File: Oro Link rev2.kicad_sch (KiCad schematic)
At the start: 18 parts, among them J1 690357100872, J10 690367180872, J11 690367180872, J12 690367180872, J13 690367180872, J14 690357100872, J15 690357100872, J16 690357100872, J17 690357100872, J18 690357100872, J2 690357100872, J3 690357100872, J4 690357100872, J5 690367180872, J6 690367180872, J7 690367180872, J8 690367180872, J9 690367180872

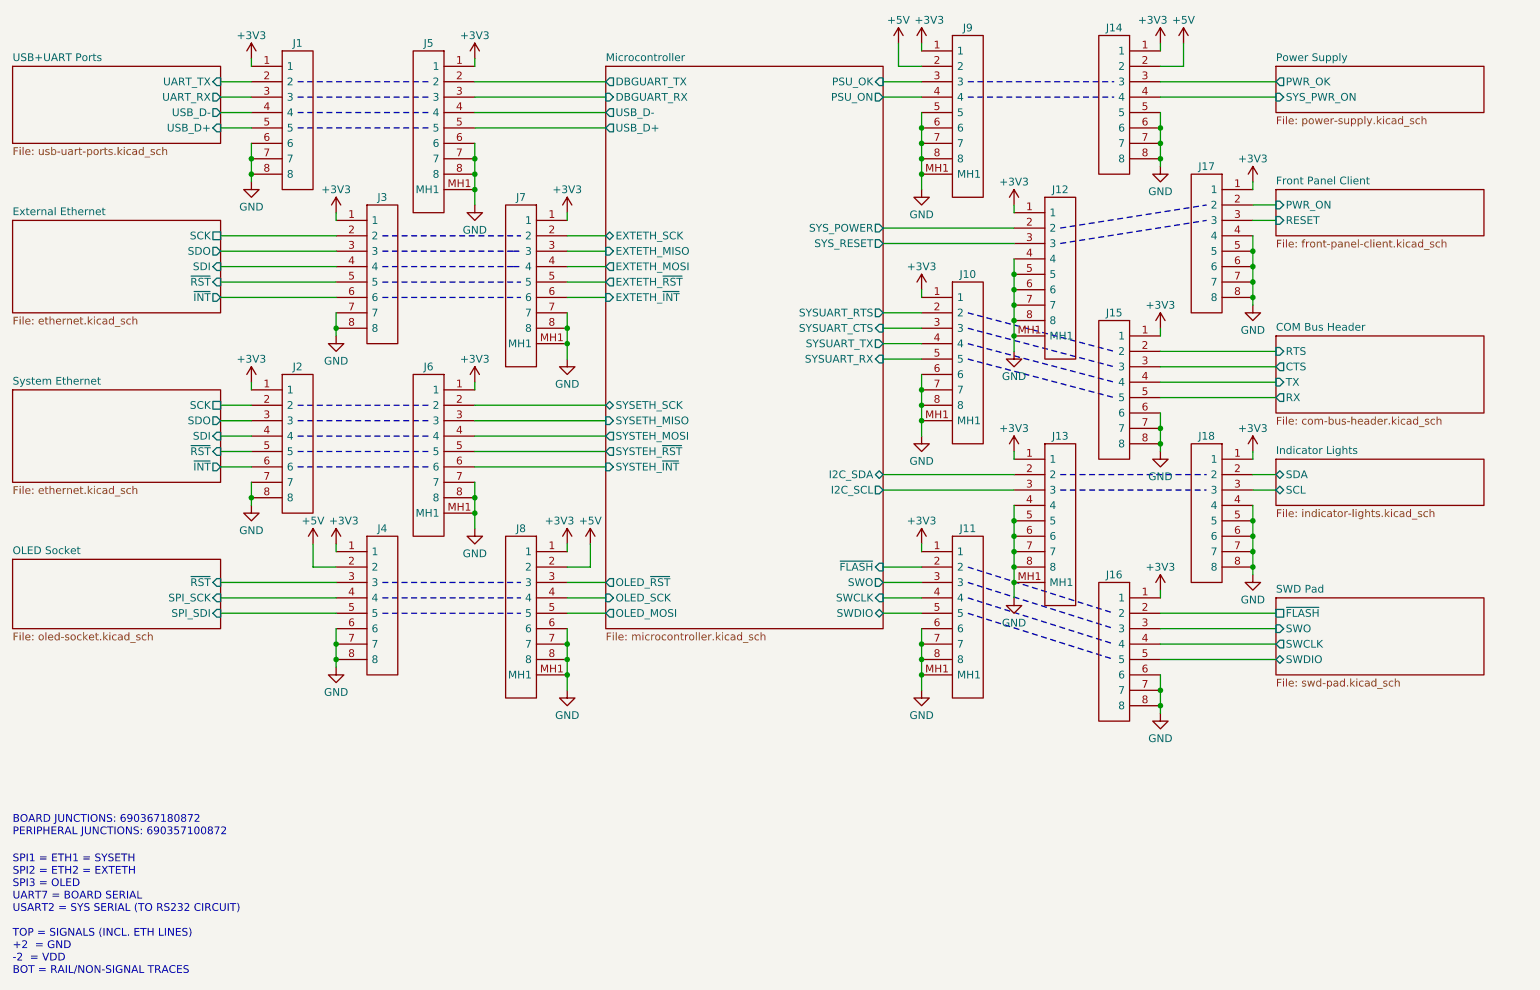
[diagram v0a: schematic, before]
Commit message: initial board layout
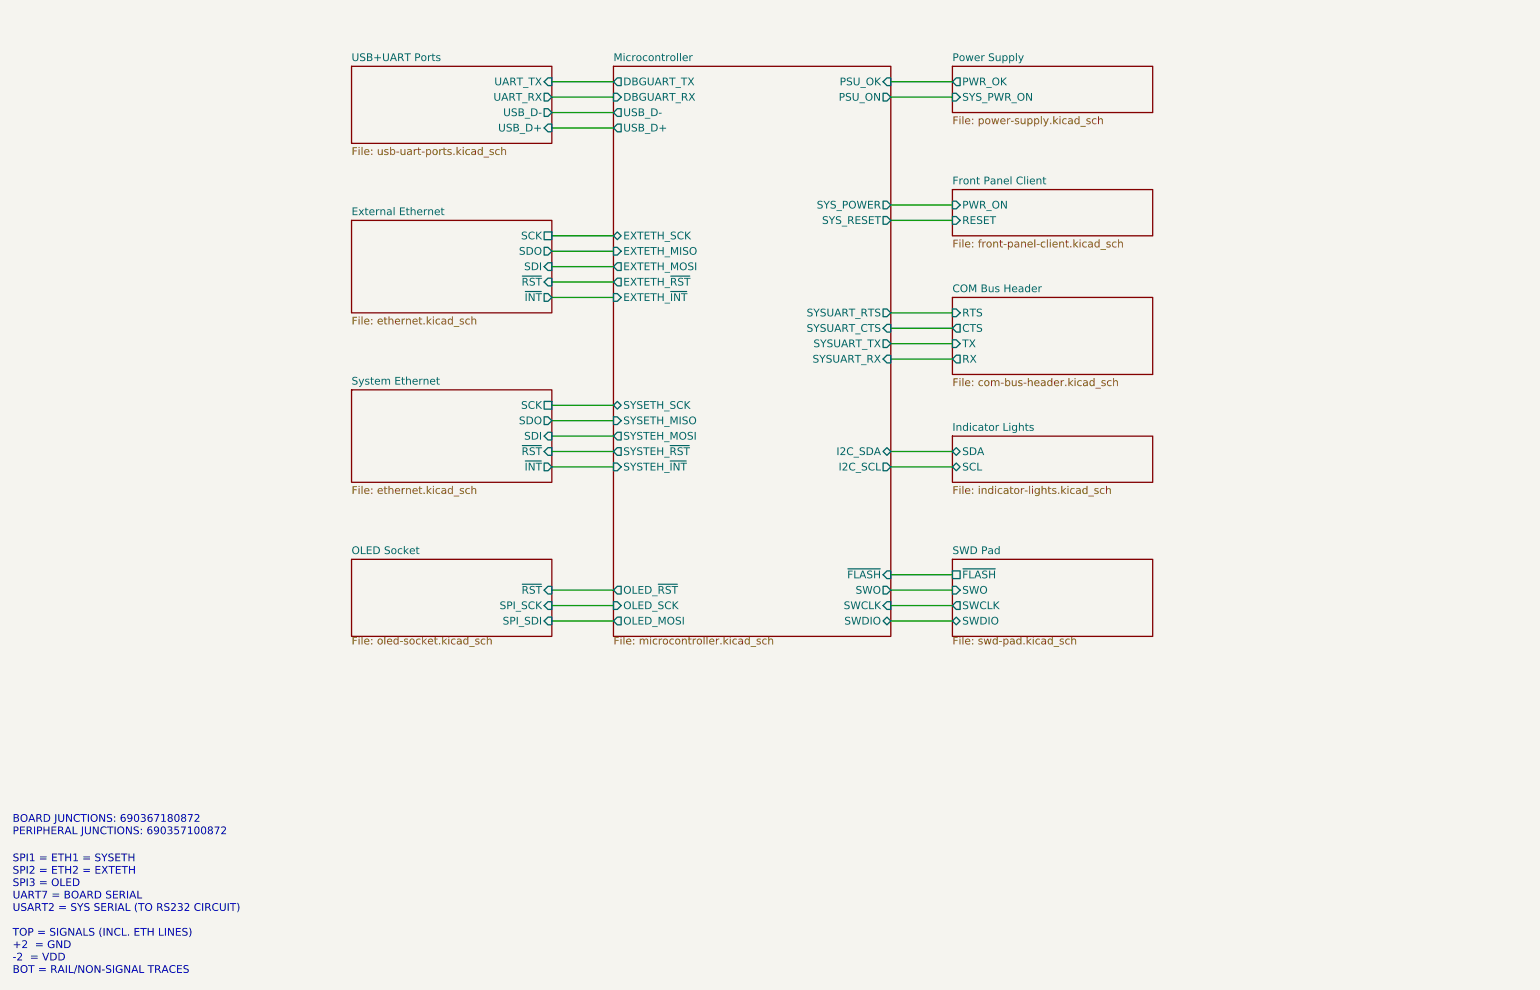
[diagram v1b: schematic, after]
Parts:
- removed J1, J14, J15, J16, J17, J18, J2, J3, J4: 690357100872, Oro Footprints:690357100872, symbol Oro:690357100872
- removed J10, J11, J12, J13, J5, J6, J7, J8, J9: 690367180872, 690367180872, symbol SamacSys_Parts:690367180872
